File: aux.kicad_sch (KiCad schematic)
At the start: 27 parts, among them J7 USB_C_Receptacle_USB2.0_16P, J85 Conn_01x02_Pin, J86 Conn_01x02_Pin, Q81 Si2301CDS, Q82 AO3400A, U85 DAC80508xRTE

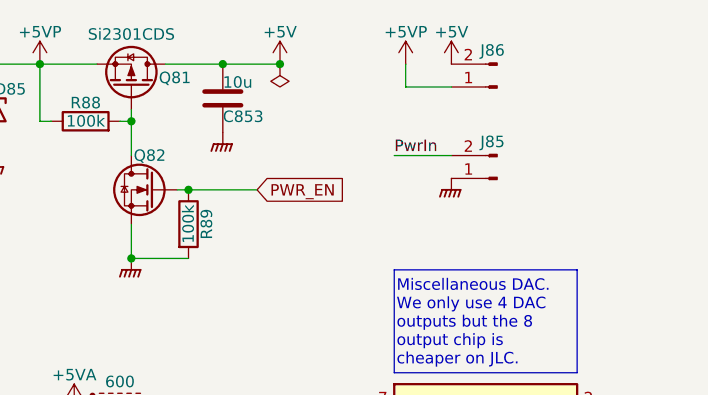
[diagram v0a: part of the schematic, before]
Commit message: Contact pads.  Shuffle the big cap.
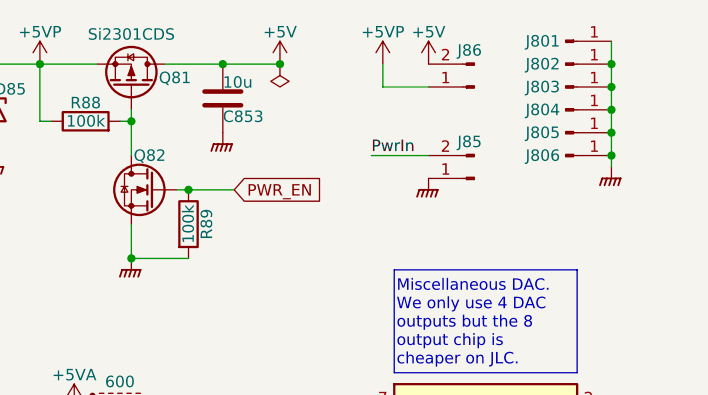
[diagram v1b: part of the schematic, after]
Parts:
- added J801, J802, J803, J804, J805, J806: Conn_01x01_Pin, Parts:RF_Finger_Side, symbol Connector:Conn_01x01_Pin
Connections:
- net GNDPWR: now also J801.1 (Pin_1), J802.1 (Pin_1), J803.1 (Pin_1), J804.1 (Pin_1), J805.1 (Pin_1), J806.1 (Pin_1)
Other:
- moved on the sheet: J85, J86
